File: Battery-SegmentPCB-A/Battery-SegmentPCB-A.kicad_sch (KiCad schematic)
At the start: 10 parts, among them J1 Conn_01x04, J10 Conn_01x09, J2 Conn_01x04, J3 Conn_01x04, J4 Conn_01x04, J5 Conn_01x04, J6 Conn_01x04, J7 Conn_01x04, J8 Conn_01x04, J9 Conn_01x09

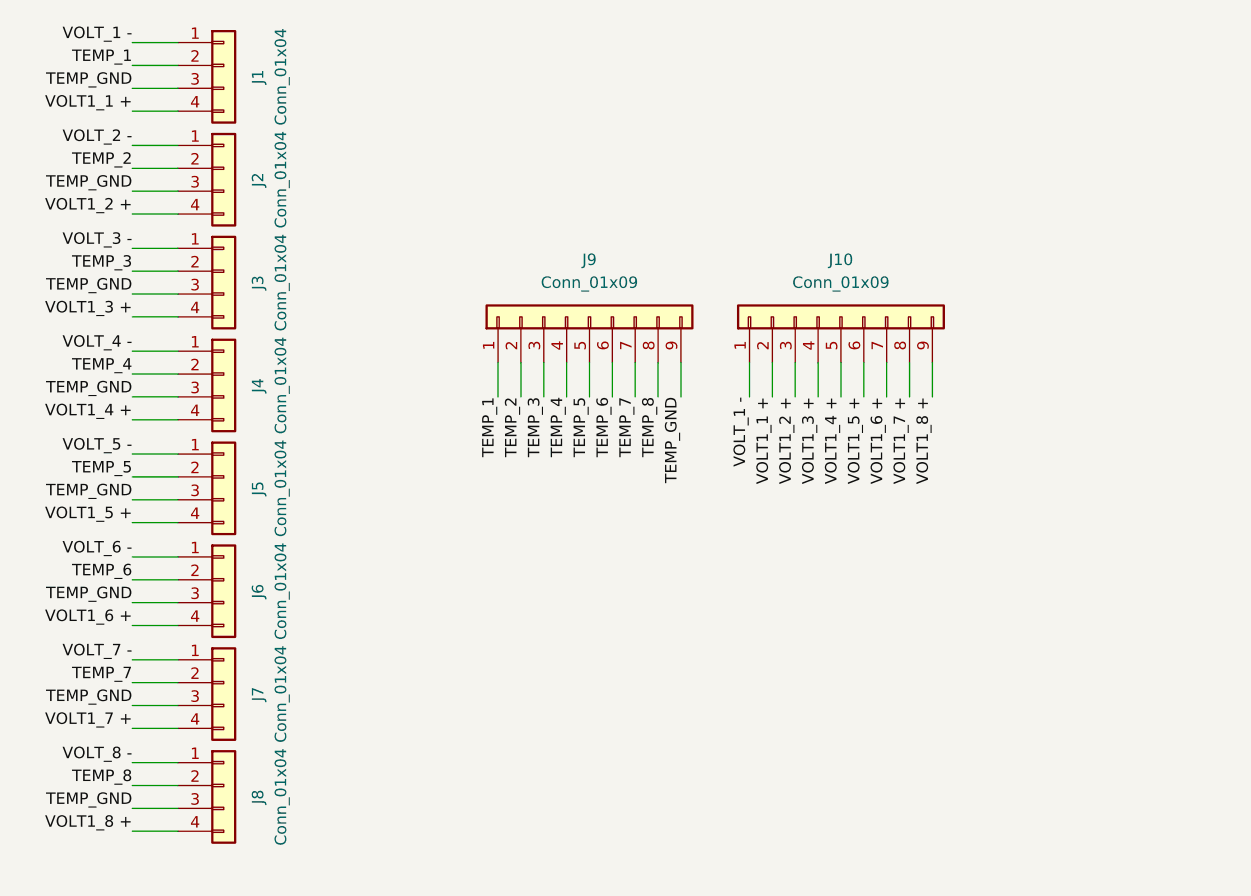
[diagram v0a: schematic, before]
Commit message: started
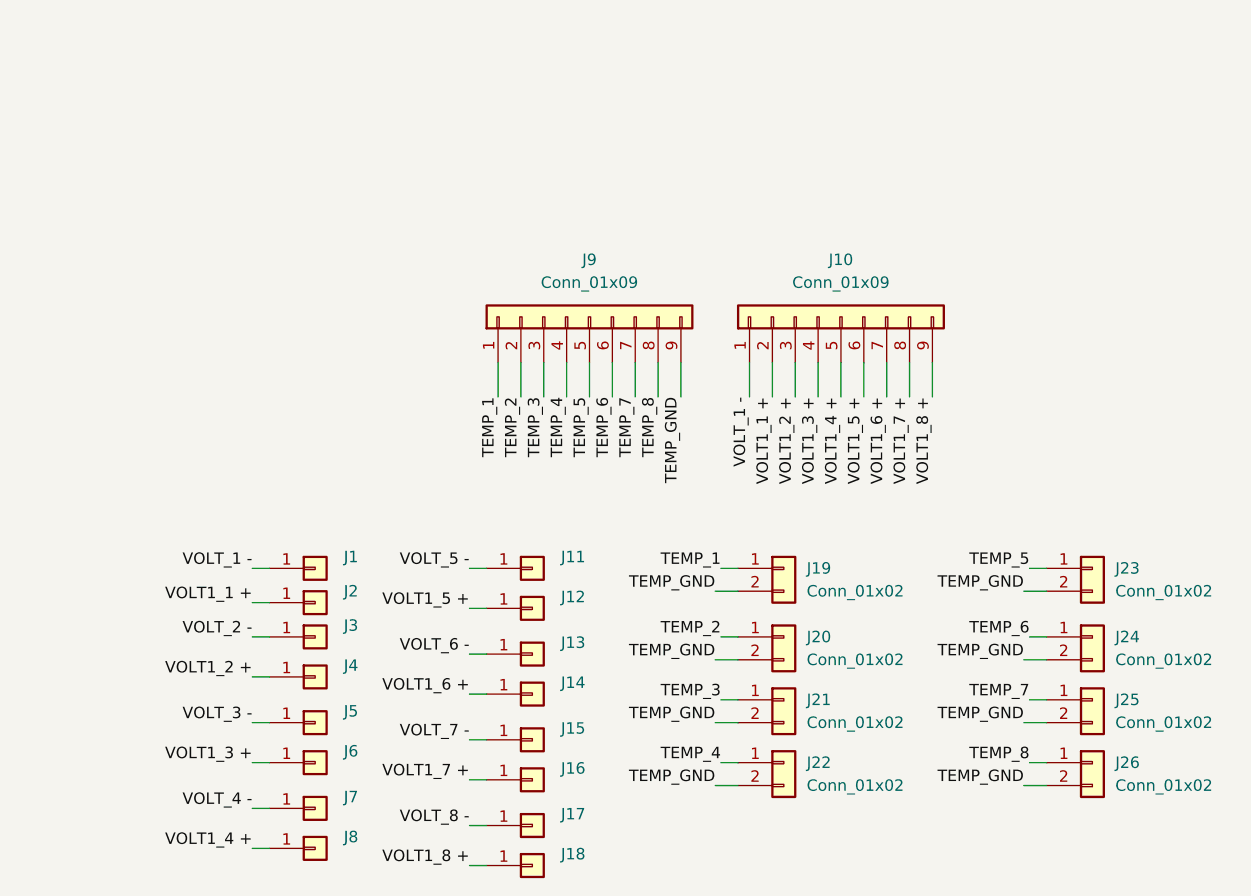
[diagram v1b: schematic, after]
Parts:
- removed J1, J2, J3, J4, J5, J6, J7, J8: Conn_01x04, footprints:CONN_S4B-PH-K-S_JST, symbol Connector_Generic:Conn_01x04
- added J1, J11, J12, J13, J14, J15, J16, J17, J18, J2, J3, J4, J5, J6, J7, J8: Conn_01x01, MountingHole:MountingHole_3.2mm_M3_DIN965_Pad_TopOnly, symbol Connector_Generic:Conn_01x01
- added J19, J20, J21, J22, J23, J24, J25, J26: Conn_01x02, Connector_Molex:Molex_Nano-Fit_105309-xx02_1x02_P2.50mm_Vertical, symbol Connector_Generic:Conn_01x02
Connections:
- net TEMP_1: now also J19.1 (Pin_1)
- net TEMP_2: now also J20.1 (Pin_1)
- net TEMP_3: now also J21.1 (Pin_1)
- net TEMP_4: now also J22.1 (Pin_1)
- net TEMP_5: now also J23.1 (Pin_1)
- net TEMP_6: now also J24.1 (Pin_1)
- net TEMP_7: now also J25.1 (Pin_1)
- net TEMP_8: now also J26.1 (Pin_1)
- net TEMP_GND: now also J19.2 (Pin_2), J20.2 (Pin_2), J21.2 (Pin_2), J22.2 (Pin_2), J23.2 (Pin_2), J24.2 (Pin_2), J25.2 (Pin_2), J26.2 (Pin_2)
- net VOLT1_1 +: now also J2.1 (Pin_1)
- net VOLT1_2 +: now also J4.1 (Pin_1)
- net VOLT1_3 +: now also J6.1 (Pin_1)
- net VOLT1_4 +: now also J8.1 (Pin_1)
- net VOLT1_5 +: now also J12.1 (Pin_1)
- net VOLT1_6 +: now also J14.1 (Pin_1)
- net VOLT1_7 +: now also J16.1 (Pin_1)
- net VOLT1_8 +: now also J18.1 (Pin_1)
- net VOLT_1 -: now also J1.1 (Pin_1)
- net VOLT_2 -: now also J3.1 (Pin_1)
- net VOLT_3 -: now also J5.1 (Pin_1)
- net VOLT_4 -: now also J7.1 (Pin_1)
- net VOLT_5 -: now also J11.1 (Pin_1)
- net VOLT_6 -: now also J13.1 (Pin_1)
- net VOLT_7 -: now also J15.1 (Pin_1)
- net VOLT_8 -: now also J17.1 (Pin_1)

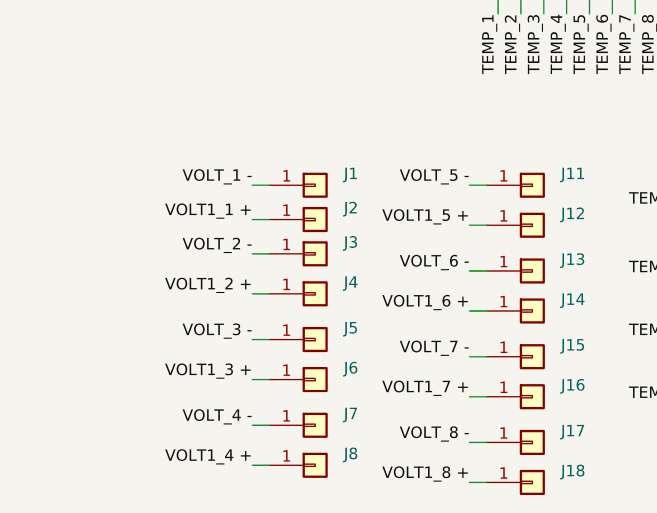
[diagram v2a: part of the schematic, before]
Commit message: stuff
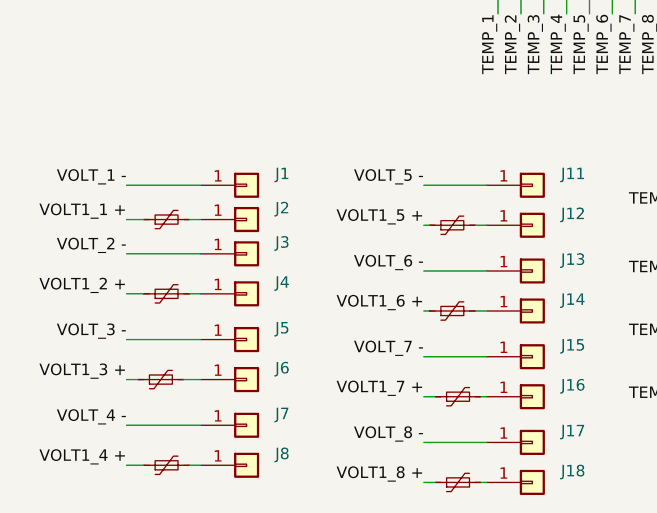
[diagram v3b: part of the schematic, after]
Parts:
- added F37, F38, F39, F40, F41, F42, F43, F44: PTC Fuse, footprints:FUSC1810X100N, symbol Device:Polyfuse_Small
- J19, J20, J21, J22, J23, J24, J25, J26: footprint Connector_Molex:Molex_Nano-Fit_105309-xx02_1x02_P2.50mm_Vertical -> UTSVT_Connectors:105313-2102
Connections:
- net VOLT1_1 +: now also F37.1; no longer J2.1 (Pin_1)
- net VOLT1_2 +: now also F38.1; no longer J4.1 (Pin_1)
- net VOLT1_3 +: now also F39.1; no longer J6.1 (Pin_1)
- net VOLT1_4 +: now also F40.1; no longer J8.1 (Pin_1)
- net VOLT1_5 +: now also F41.1; no longer J12.1 (Pin_1)
- net VOLT1_6 +: now also F42.1; no longer J14.1 (Pin_1)
- net VOLT1_7 +: now also F43.1; no longer J16.1 (Pin_1)
- net VOLT1_8 +: now also F44.1; no longer J18.1 (Pin_1)
- new net: F44.2, J18.1 (Pin_1)
- new net: F37.2, J2.1 (Pin_1)
- new net: F38.2, J4.1 (Pin_1)
- new net: F39.2, J6.1 (Pin_1)
- new net: F41.2, J12.1 (Pin_1)
- new net: F42.2, J14.1 (Pin_1)
- new net: F43.2, J16.1 (Pin_1)
- new net: F40.2, J8.1 (Pin_1)
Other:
- moved on the sheet: J1, J2, J3, J4, J5, J6, J7, J8
